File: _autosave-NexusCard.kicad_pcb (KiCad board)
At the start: 2 copper layers, 3 parts, among them U1 NCP1117-1.5_SOT223, U2 W25Q128JVS, U3 RP2040

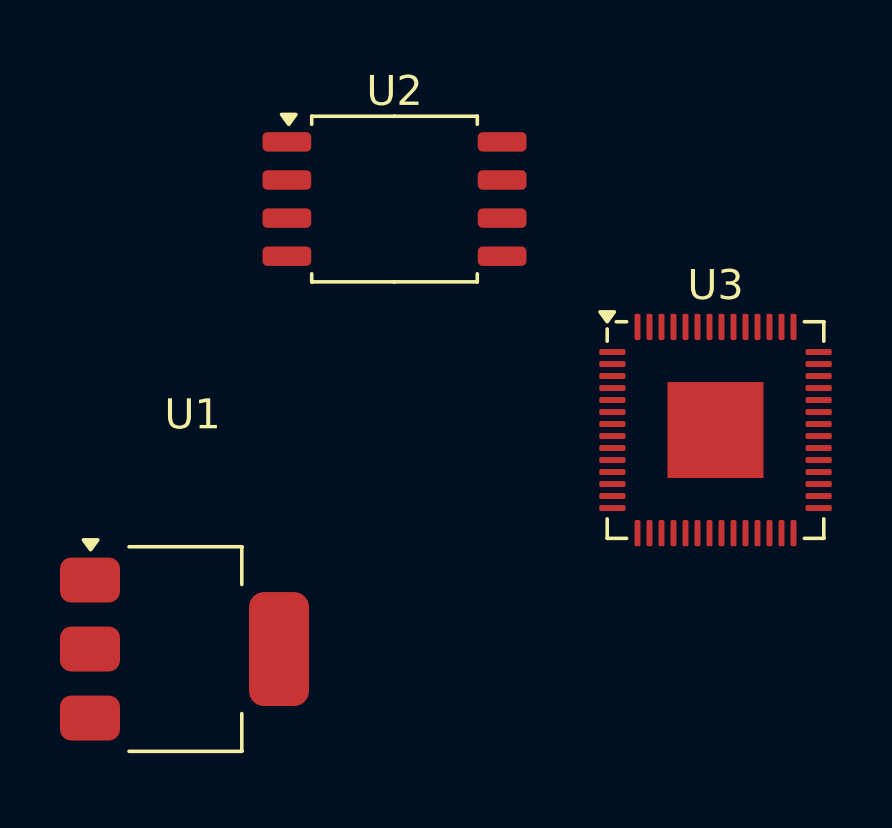
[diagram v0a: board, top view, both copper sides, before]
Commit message: it aint much but honest work
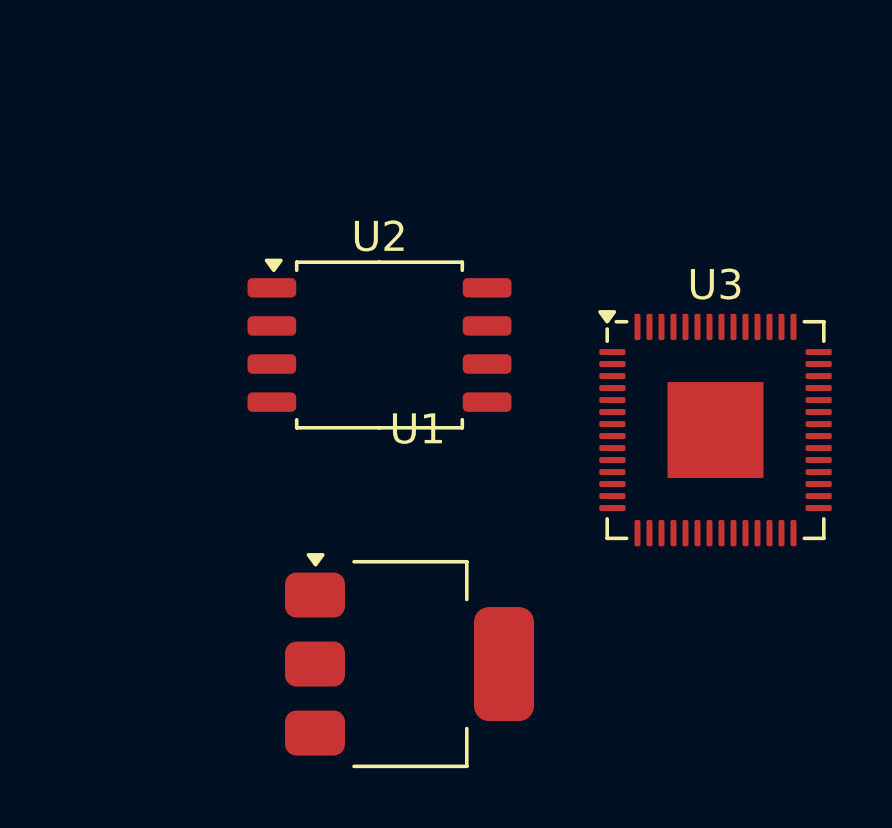
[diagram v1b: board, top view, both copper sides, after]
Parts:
- moved U1 7.52 mm to (150.5, 98.0)
- moved U2 4.89 mm to (149.5, 87.4)
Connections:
- U3 pad 19: unconnected-(U3-TESTEN-Pad19) -> GND
- U3 pad 20: unconnected-(U3-XIN-Pad20) -> /XIN
- U3 pad 21: unconnected-(U3-XOUT-Pad21) -> /XOUT
- U3 pad 46: unconnected-(U3-USB_DM-Pad46) -> Net-(U3-USB_DM)
- U3 pad 47: unconnected-(U3-USB_DP-Pad47) -> Net-(U3-USB_DP)
- U3 pad 51: unconnected-(U3-QSPI_SD3-Pad51) -> /QSPI_SD3
- U3 pad 52: unconnected-(U3-QSPI_SCLK-Pad52) -> /QSPI_SCLK
- U3 pad 53: unconnected-(U3-QSPI_SD0-Pad53) -> /QSPI_SD0
- U3 pad 54: unconnected-(U3-QSPI_SD2-Pad54) -> /QSPI_SD2
- U3 pad 55: unconnected-(U3-QSPI_SD1-Pad55) -> /QSPI_SD1
- U3 pad 56: unconnected-(U3-QSPI_SS-Pad56) -> /QSPI_SS
- U3 pad 57: unconnected-(U3-GND-Pad57) -> GND
